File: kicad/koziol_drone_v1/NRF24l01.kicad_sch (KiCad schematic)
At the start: 1 part, among them U5 NRF24L01

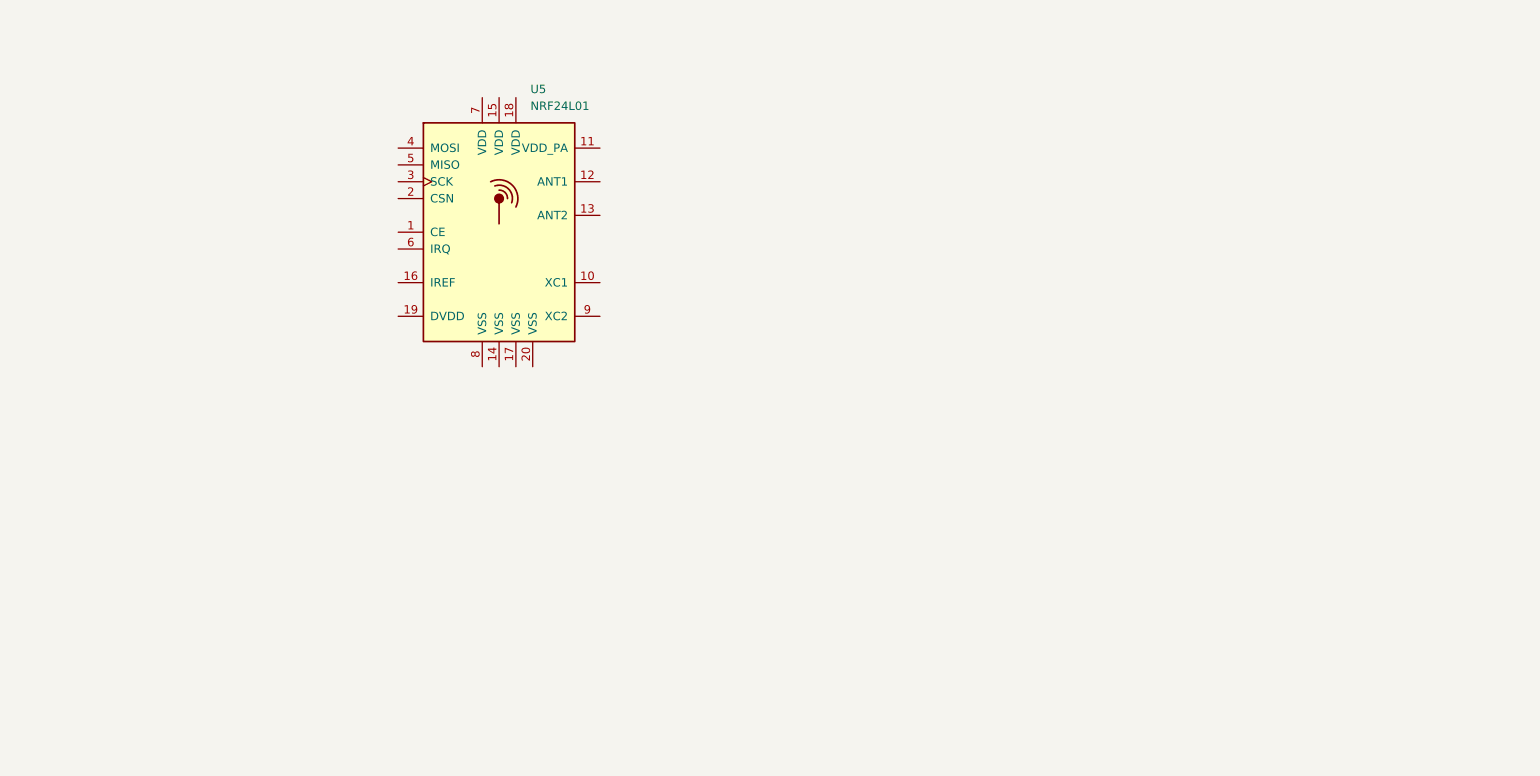
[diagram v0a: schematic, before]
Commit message: schemes progress
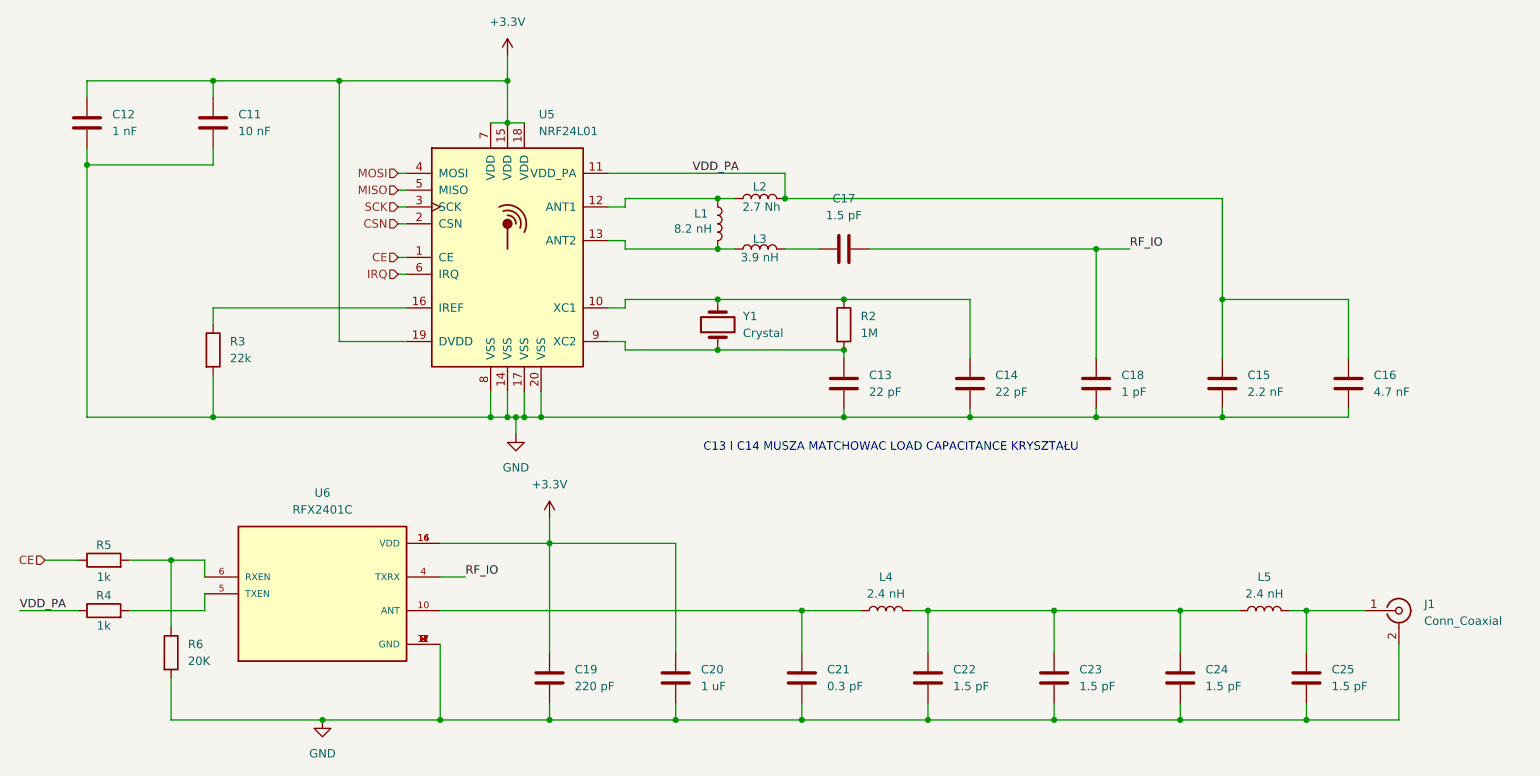
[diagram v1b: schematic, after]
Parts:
- added C11: 10 nF, symbol Device:C
- added C12: 1 nF, symbol Device:C
- added C13, C14: 22 pF, symbol Device:C
- added C15: 2.2 nF, symbol Device:C
- added C16: 4.7 nF, symbol Device:C
- added C17, C22, C23, C24, C25: 1.5 pF, symbol Device:C
- added C18: 1 pF, symbol Device:C
- added C19: 220 pF, symbol Device:C
- added C20: 1 uF, symbol Device:C
- added C21: 0.3 pF, symbol Device:C
- added J1: Conn_Coaxial, Connector_Coaxial:SMA_Amphenol_901-143_Horizontal, symbol Connector:Conn_Coaxial
- added L1: 8.2 nH, symbol Device:L
- added L2: 2.7 Nh, symbol Device:L
- added L3: 3.9 nH, symbol Device:L
- added L4, L5: 2.4 nH, symbol Device:L
- added R2: 1M, symbol Device:R
- added R3: 22k, symbol Device:R
- added R4, R5: 1k, symbol Device:R
- added R6: 20K, symbol Device:R
- added U6: RFX2401C, RFX2401C:QFN50P300X300X60-17N, symbol RFX2401C:RFX2401C
- added Y1: Crystal, symbol Device:Crystal
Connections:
- net CE: now reaches U5.1 (CE)
- net CE: now also R5.1
- net at U5.10 (XC1): now also C14.1, R2.1, Y1.2
- net VDD_PA: now reaches U5.11 (VDD_PA)
- net VDD_PA: now also C15.1, C16.1, L2.2, R4.1
- net at U5.12 (ANT1): now also L1.1, L2.1
- net at U5.13 (ANT2): now also L1.2, L3.1
- net GND: now reaches U5.14 (VSS)
- net GND: now also U5.17 (VSS), U5.20 (VSS), U5.8 (VSS), C11.2, C12.2, C13.2, C14.2, C15.2, C16.2, C18.1, C19.2, C20.2, C21.2, C22.2, C23.2, C24.2, C25.2, J1.2 (Ext), R3.2, R6.2, U6.11 (GND), U6.17 (GND), U6.2 (GND), U6.3 (GND), U6.8 (GND), U6.9 (GND)
- net +3.3V: now reaches U5.15 (VDD)
- net +3.3V: now also U5.18 (VDD), U5.19 (DVDD), U5.7 (VDD), C11.1, C12.1, C19.1, C20.1, U6.14 (VDD), U6.16 (VDD)
- net at U5.16 (IREF): now also R3.1
- net CSN: now reaches U5.2 (CSN)
- net SCK: now reaches U5.3 (SCK)
- net MOSI: now reaches U5.4 (MOSI)
- net MISO: now reaches U5.5 (MISO)
- net IRQ: now reaches U5.6 (IRQ)
- net at U5.9 (XC2): now also C13.1, R2.2, Y1.1
- new net: C25.1, J1.1 (In), L5.2
- new net: C22.1, C23.1, C24.1, L4.2, L5.1
- new net: C17.1, L3.2
- new net: R5.2, R6.1, U6.6 (RXEN)
- new net: R4.2, U6.5 (TXEN)
- new net: C21.1, L4.1, U6.10 (ANT)
- new net RF_IO: C17.2, C18.2, U6.4 (TXRX)
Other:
- note added: "C13 I C14 MUSZA MATCHOWAC LOAD CAPACITANCE KRYSZTAŁU"
- moved on the sheet: U5
